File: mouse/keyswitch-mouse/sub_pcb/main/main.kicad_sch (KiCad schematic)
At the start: 28 parts, among them J1 USB_C_Receptacle_USB2.0_16P, J2 Conn_01x02_Socket, SW1 Switch, U1 USB6B1, U2 USBLC6-2SC6, U3 nRF52840, U4 MCP73831-2-OT, Y2 Crystal_GND3

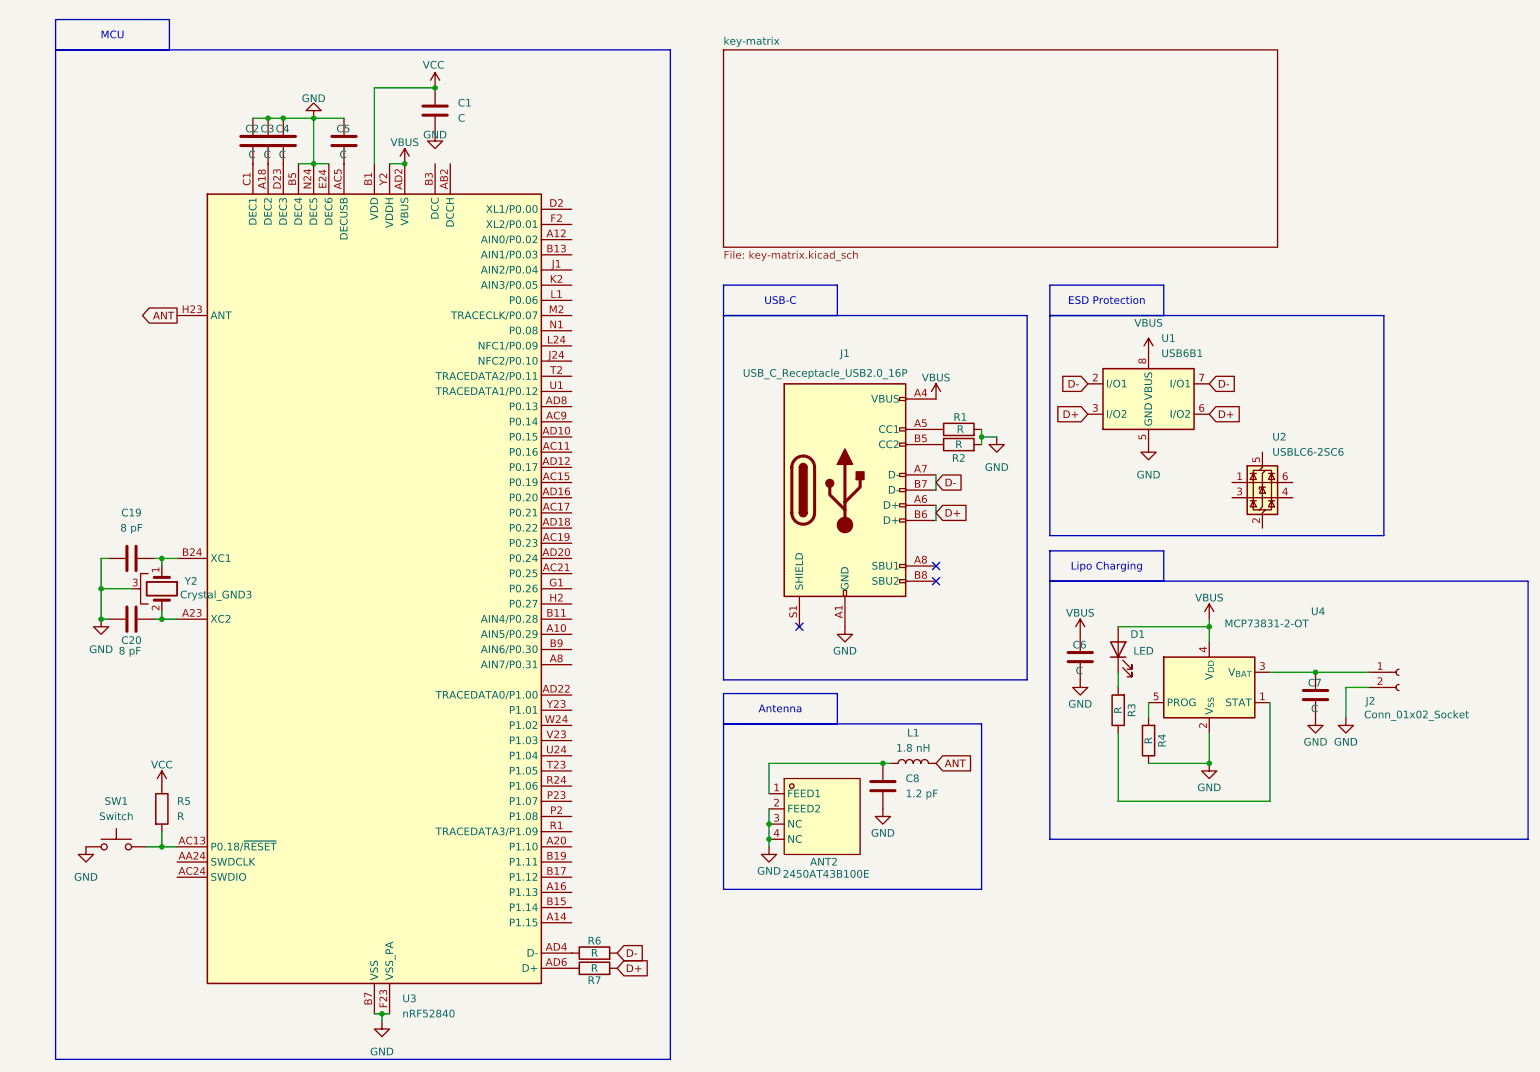
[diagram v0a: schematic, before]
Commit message: 1:31am 4-28-25
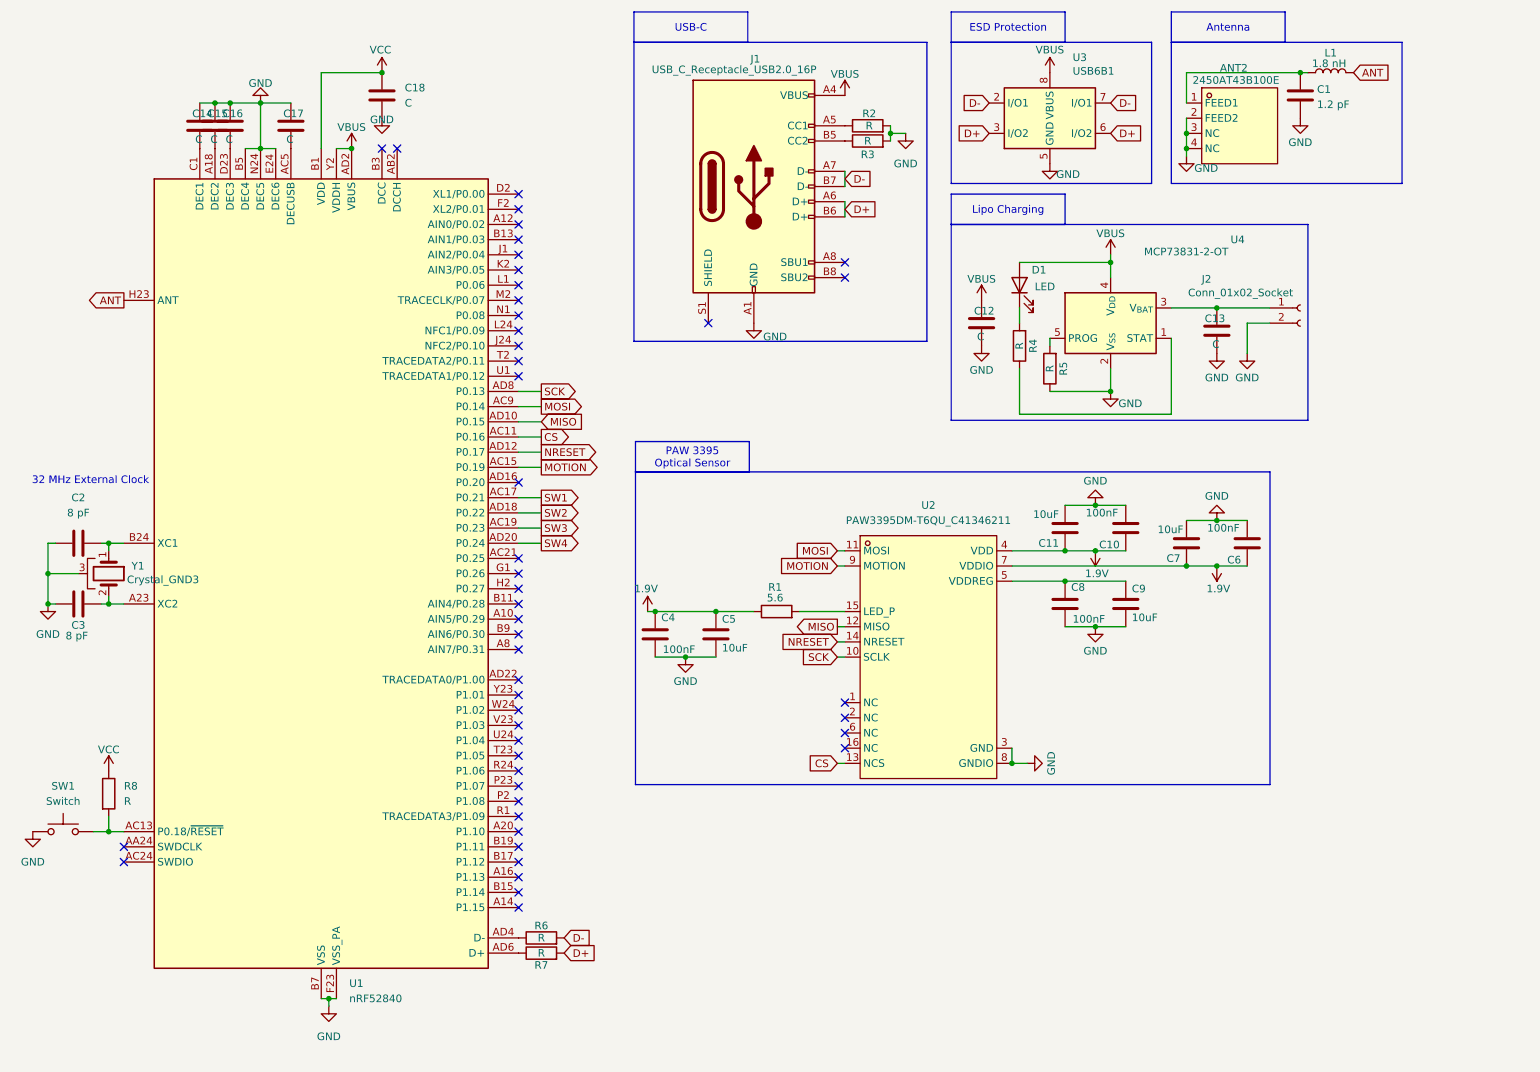
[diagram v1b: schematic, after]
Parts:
- removed C19, C20: 8 pF, symbol Device:C
- removed R5: R, symbol Device:R
- removed U1: USB6B1, Package_SO:SOIC-8_3.9x4.9mm_P1.27mm, symbol Power_Protection:USB6B1
- removed U2: USBLC6-2SC6, Package_TO_SOT_SMD:SOT-23-6, symbol Power_Protection:USBLC6-2SC6
- removed U3: nRF52840, Package_DFN_QFN:Nordic_AQFN-73-1EP_7x7mm_P0.5mm, symbol MCU_Nordic:nRF52840
- removed Y2: Crystal_GND3, symbol Device:Crystal_GND3
- added C10: 100nF, symbol Device:C
- added C11, C9: 10uF, symbol Device:C
- added C12, C13, C14, C15, C16, C17, C18: C, symbol Device:C
- added R2, R8: R, symbol Device:R
- added U1: nRF52840, Package_DFN_QFN:Nordic_AQFN-73-1EP_7x7mm_P0.5mm, symbol MCU_Nordic:nRF52840
- added U2: PAW3395DM-T6QU_C41346211, easyeda2kicad:PDIP-16_L16.2-W9.1-P1.78-TL_PMW3389DM-T3QU, symbol easyeda2kicad:PAW3395DM-T6QU_C41346211
- added U3: USB6B1, Package_SO:SOIC-8_3.9x4.9mm_P1.27mm, symbol Power_Protection:USB6B1
- added Y1: Crystal_GND3, symbol Device:Crystal_GND3
- C1: value C -> 1.2 pF
- C2, C3: value C -> 8 pF
- C4, C6: value C -> 100nF
- C5, C7: value C -> 10uF
- C8: value 1.2 pF -> 100nF
- R1: value R -> 5.6
- renumbered R2 to R3, R3 to R4, R4 to R5
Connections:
- net ANT: now also U1.H23 (ANT)
- net D+: now also U3.3 (I/O2), U3.6 (I/O2)
- net D-: now also U3.2 (I/O1), U3.7 (I/O1)
- net GND: now also C4.2, C5.2, C10.2, C11.2, C12.2, C13.2, C14.1, C15.1, C16.1, C17.1, C18.2, C9.2, R2.2, U1.B5 (DEC4), U1.B7 (VSS), U1.E24 (DEC6), U1.EP (VSS), U1.F23 (VSS_PA), U1.N24 (DEC5), U2.3 (GND), U2.8 (GNDIO), U3.4 (GND), U3.5 (GND), Y1.3; no longer C4.1, C5.1, R1.2
- net VBUS: now also C12.1, U1.AD2 (VBUS), U1.Y2 (VDDH), U3.1 (VBUS), U3.8 (VBUS); no longer C6.1
- net VCC: now also C18.1, R8.1, U1.A22 (VDD), U1.AD14 (VDD), U1.AD23 (VDD), U1.B1 (VDD), U1.W1 (VDD); no longer C1.1
- net at C3.2: now also U1.A23 (XC2), Y1.2
- net at SW1.2: now also R8.2, U1.AC13 (P0.18/~{RESET})
- net at ANT2.1 (FEED1), L1.1: now also C1.1; no longer C8.1
- net at R6.1: now also U1.AD4 (D-)
- net at J2.1 (Pin_1), U4.3 (V_{BAT}): now also C13.1; no longer C7.1
- net at R7.1: now also U1.AD6 (D+)
- net at C2.2: now also U1.B24 (XC1), Y1.1
- net at J1.A5 (CC1): now also R2.1; no longer R1.1
- new net: C16.2, U1.D23 (DEC3)
- new net: C8.1, C9.1, U2.5 (VDDREG)
- new net: C17.2, U1.AC5 (DECUSB)
- new net: R1.2, U2.15 (LED_P)
- new net: C15.2, U1.A18 (DEC2)
- new net: C14.2, U1.C1 (DEC1)
- new net 1.9V: C10.1, C11.1, C4.1, C5.1, C6.1, C7.1, R1.1, U2.4 (VDD), U2.7 (VDDIO)
- new net CS: U1.AC11 (P0.16), U2.13 (NCS)
- new net MISO: U1.AD10 (P0.15), U2.12 (MISO)
- new net MOSI: U1.AC9 (P0.14), U2.11 (MOSI)
- new net MOTION: U1.AC15 (P0.19), U2.9 (MOTION)
- new net NRESET: U1.AD12 (P0.17), U2.14 (NRESET)
- new net SCK: U1.AD8 (P0.13), U2.10 (SCLK)
- new net SW1: U1.AC17 (P0.21)
- new net SW2: U1.AD18 (P0.22)
- new net SW3: U1.AC19 (P0.23)
- new net SW4: U1.AD20 (P0.24)
- no-connect marks 3 -> 48
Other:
- removed sheet key-matrix
- note added: "32 MHz External Clock"
- moved on the sheet: ANT2, D1, J1, J2, L1, R3, R4, R5, R6, R7, SW1, U4
